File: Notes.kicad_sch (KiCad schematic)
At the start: 0 parts

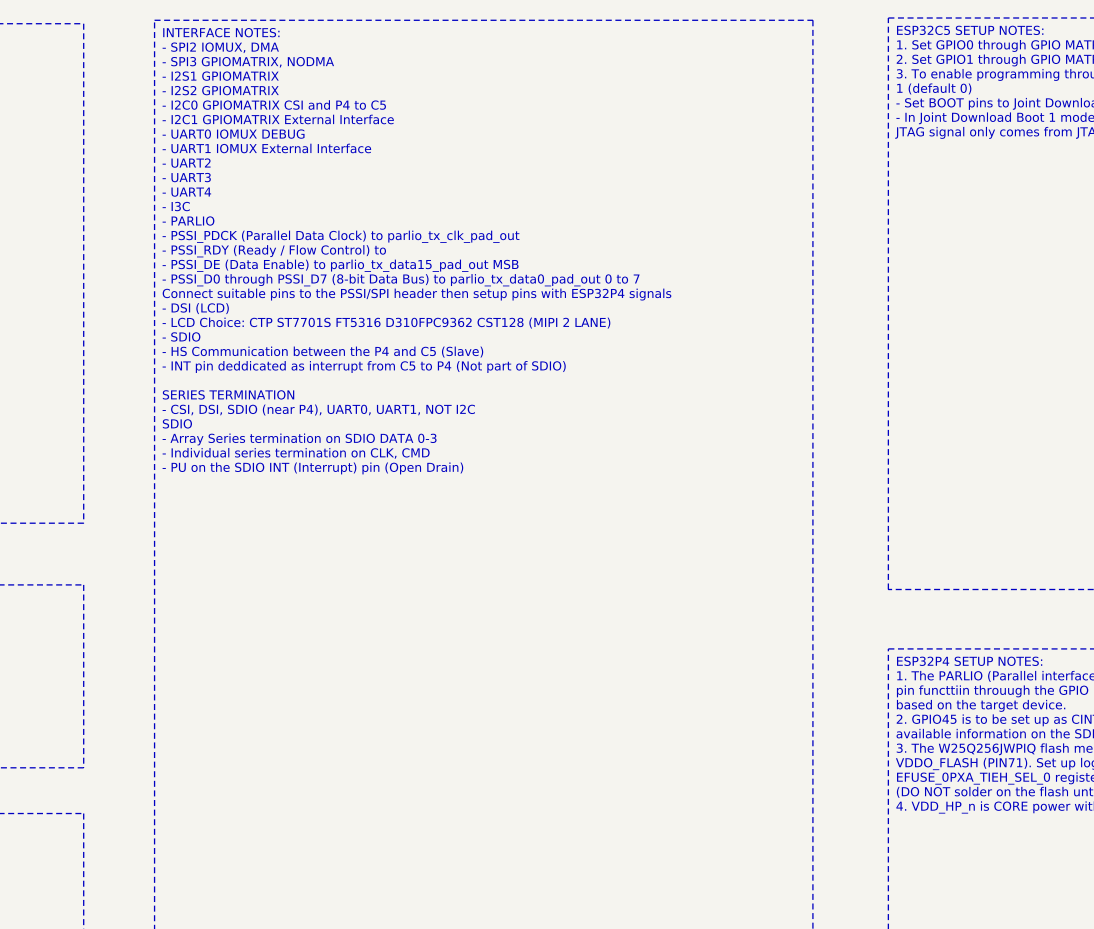
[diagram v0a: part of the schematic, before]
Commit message: SMA Update
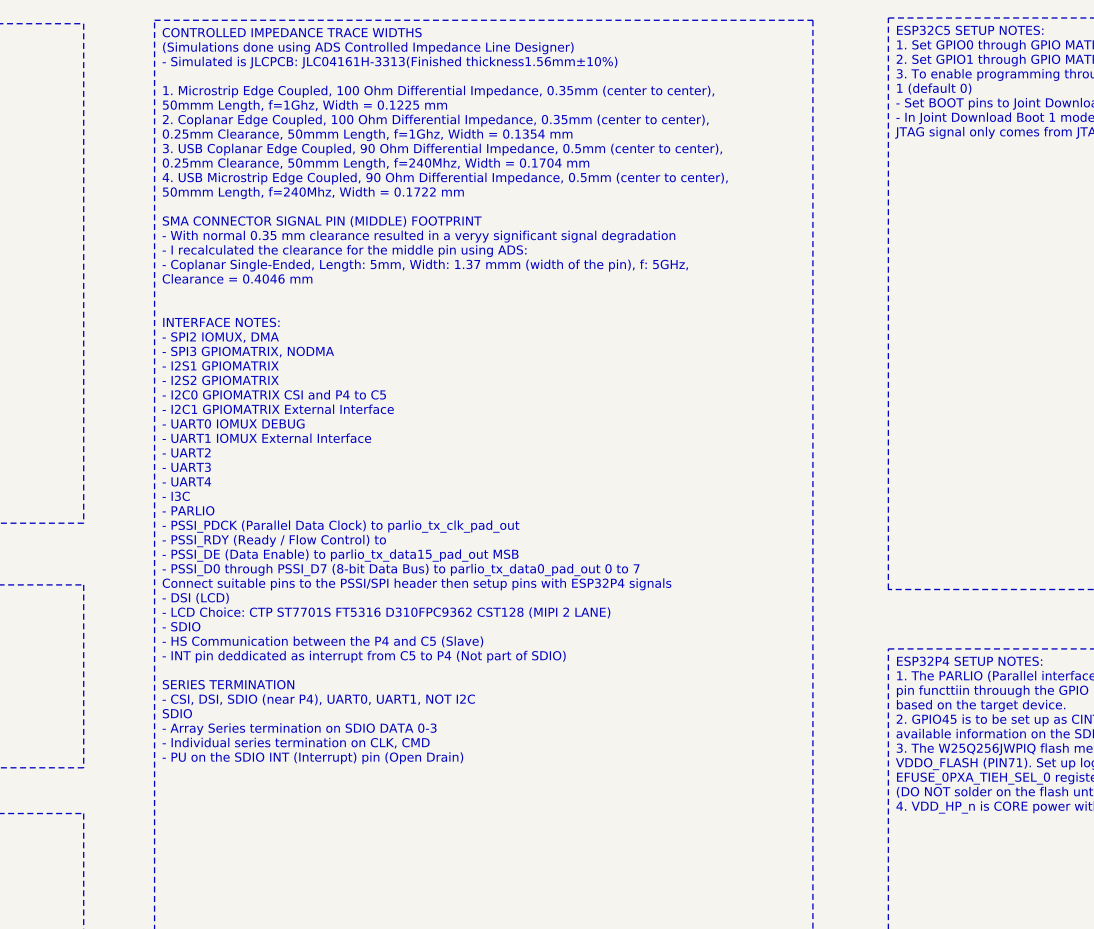
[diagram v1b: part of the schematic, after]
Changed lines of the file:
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@@
 	(generator_version "8.0")
 	(paper "A4")
-	(text_box "INTERFACE NOTES:\n- SPI2 IOMUX, DMA\n- SPI3 GPIOMATRIX, NODMA\n- I2S1 GPIOMATRIX\n- I2S2 GPIOMATRIX\n- I2C0 GPIOMATRIX CSI and P4 to C5\n- I2C1 GPIOMATRIX External Interface\n- UART0 IOMUX DEBUG\n- UART1 IOMUX External Interface\n- UART2\n- UART3\n- UART4\n- I3C\n- PARLIO\n  - PSSI_PDCK (Parallel Data Clock) to parlio_tx_clk_pad_out\n  - PSSI_RDY (Ready / Flow Control) to \n  - PSSI_DE (Data Enable) to parlio_tx_data15_pad_out MSB\n  - PSSI_D0 through PSSI_D7 (8-bit Data Bus) to parlio_tx_data0_pad_out 0 to 7\n  Connect suitable pins to the PSSI/SPI header then setup pins with ESP32P4 signals\n- DSI (LCD)\n  - LCD Choice: CTP ST7701S FT5316 D310FPC9362 CST128 (MIPI 2 LANE)\n- SDIO\n  - HS Communication between the P4 and C5 (Slave)\n  - INT pin deddicated as interrupt from C5 to P4 (Not part of SDIO)\n\nSERIES TERMINATION\n- CSI, DSI, SDIO (near P4), UART0, UART1, NOT I2C\nSDIO\n- Array Series termination on SDIO DATA 0-3\n- Individual series termination on CLK, CMD\n- PU on the SDIO INT (Interrupt) pin (Open Drain)"
+	(text_box "CONTROLLED IMPEDANCE TRACE WIDTHS\n(Simulations done using ADS Controlled Impedance Line Designer)\n- Simulated is JLCPCB: JLC04161H-3313(Finished thickness1.56mm±10%)\n\n1. Microstrip Edge Coupled, 100 Ohm Differential Impedance, 0.35mm (center to center), 50mmm Length, f=1Ghz, Width = 0.1225 mm\n2. Coplanar Edge Coupled, 100 Ohm Differential Impedance, 0.35mm (center to center), 0.25mm Clearance, 50mmm Length, f=1Ghz, Width = 0.1354 mm\n3. USB Coplanar Edge Coupled, 90 Ohm Differential Impedance, 0.5mm (center to center), 0.25mm Clearance, 50mmm Length, f=240Mhz, Width = 0.1704 mm\n4. USB Microstrip Edge Coupled, 90 Ohm Differential Impedance, 0.5mm (center to center), 50mmm Length, f=240Mhz, Width = 0.1722 mm\n\nSMA CONNECTOR SIGNAL PIN (MIDDLE) FOOTPRINT\n- With normal 0.35 mm clearance resulted in a veryy significant signal degradation\n- I recalculated the clearance for the middle pin using ADS:\n  - Coplanar Single-Ended, Length: 5mm, Width: 1.37 mmm (width of the pin), f: 5GHz, Clearance = 0.4046 mm\n  \n\nINTERFACE NOTES:\n- SPI2 IOMUX, DMA\n- SPI3 GPIOMATRIX, NODMA\n- I2S1 GPIOMATRIX\n- I2S2 GPIOMATRIX\n- I2C0 GPIOMATRIX CSI and P4 to C5\n- I2C1 GPIOMATRIX External Interface\n- UART0 IOMUX DEBUG\n- UART1 IOMUX External Interface\n- UART2\n- UART3\n- UART4\n- I3C\n- PARLIO\n  - PSSI_PDCK (Parallel Data Clock) to parlio_tx_clk_pad_out\n  - PSSI_RDY (Ready / Flow Control) to \n  - PSSI_DE (Data Enable) to parlio_tx_data15_pad_out MSB\n  - PSSI_D0 through PSSI_D7 (8-bit Data Bus) to parlio_tx_data0_pad_out 0 to 7\n  Connect suitable pins to the PSSI/SPI header then setup pins with ESP32P4 signals\n- DSI (LCD)\n  - LCD Choice: CTP ST7701S FT5316 D310FPC9362 CST128 (MIPI 2 LANE)\n- SDIO\n  - HS Communication between the P4 and C5 (Slave)\n  - INT pin deddicated as interrupt from C5 to P4 (Not part of SDIO)\n\nSERIES TERMINATION\n- CSI, DSI, SDIO (near P4), UART0, UART1, NOT I2C\nSDIO\n- Array Series termination on SDIO DATA 0-3\n- Individual series termination on CLK, CMD\n- PU on the SDIO INT (Interrupt) pin (Open Drain)"
 		(exclude_from_sim no)
 		(at 113.03 29.464 0)
